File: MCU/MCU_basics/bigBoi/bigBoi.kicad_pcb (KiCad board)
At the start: 2 copper layers, 70 x 70 mm, 90 parts, among them IC1 BMP390, J1 Conn_Coaxial, J2 Conn_Coaxial, J3 DM3AT-SF-PEJM5_40_, J4 Conn_01x05, J5 Conn_01x04, J6 Conn_01x06, J7 USB_B_Micro, SW1 Boot Switch, U1 STM32F469NIHx, U2 LT1963AxST-3.3, U3 SX1276, U5 MIA-M10Q, U6 BNO086, Y1 8MHz, Y3 32kHz

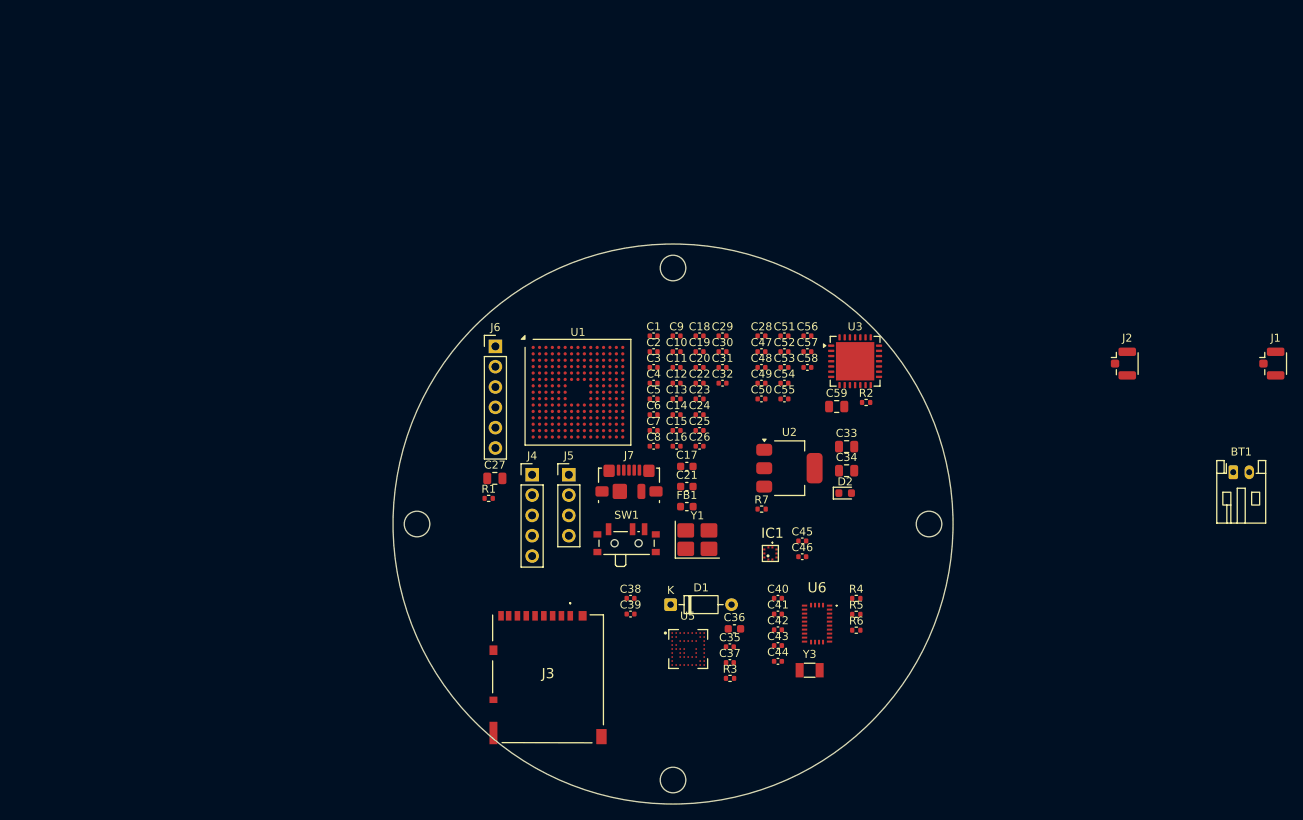
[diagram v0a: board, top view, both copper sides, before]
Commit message: Via escape routing
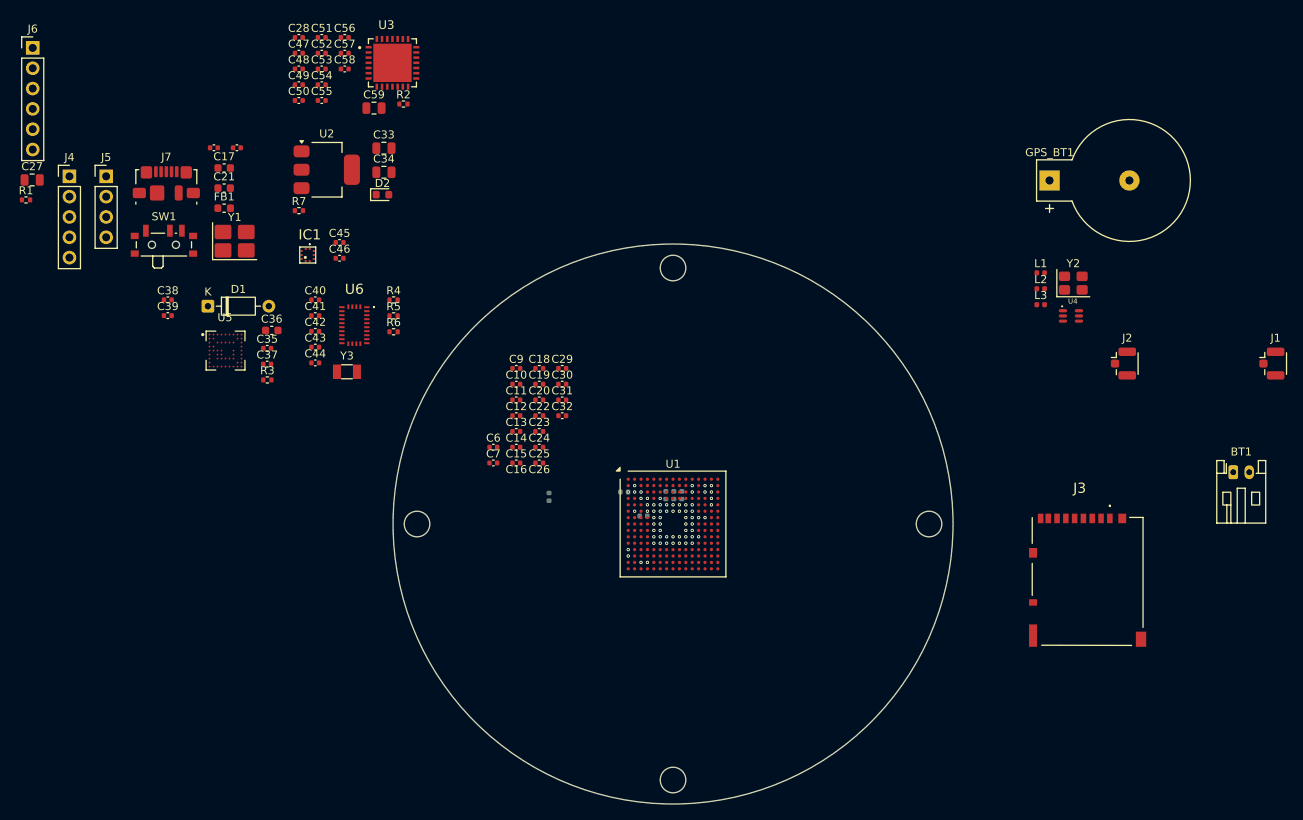
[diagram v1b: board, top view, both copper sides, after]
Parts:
- added GPS_BT1: CR1220, Battery:BatteryHolder_Keystone_500, F.Cu at (155.1, 57.1)
- added L1: 10nH, Inductor_SMD:L_0402_1005Metric, F.Cu at (154.0, 68.6)
- added L2: 10nH, Inductor_SMD:L_0402_1005Metric, F.Cu at (154.0, 70.6)
- added L3: 6.2nH, Inductor_SMD:L_0402_1005Metric, F.Cu at (154.0, 72.6)
- added U4: PE4259, Nebula-footprints:SOT65P215X110-6N, F.Cu at (157.7, 74.0)
- added Y2: 32MHz, Crystal:Crystal_SMD_3225-4Pin_3.2x2.5mm, F.Cu at (158.0, 69.9)
- C1, C2, C3, C4, C5, C8: moved to B.Cu
- C14, C18: value 0402 -> 15pF
- U3: footprint Package_DFN_QFN:QFN-28-1EP_6x6mm_P0.65mm_EP4.8x4.8mm -> Nebula-footprints:QFN65P600X600X100-29N
- moved C28 68.8 mm to (61.2, 39.2)
- moved C47 68.8 mm to (61.2, 41.1)
- moved C48 68.8 mm to (61.2, 43.1)
- moved C56 68.8 mm to (67.0, 39.2)
- moved C57 68.8 mm to (67.0, 41.1)
- moved C58 68.8 mm to (67.0, 43.1)
- moved C59 68.8 mm to (70.6, 48.0)
- moved J4 68.8 mm to (32.5, 56.5)
- moved R4 68.8 mm to (73.1, 72.0)
- moved R6 68.8 mm to (73.1, 76.0)
- moved Y1 68.8 mm to (53.2, 64.6)
- moved Y3 68.8 mm to (67.2, 81.0)
- moved C16 68.8 mm to (50.6, 53.0)
- moved C17 68.8 mm to (51.9, 55.5)
- moved C26 68.8 mm to (53.5, 53.0)
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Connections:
- J3 pad 6: <NO NET> -> GND
- J3 pad MP1: <NO NET> -> GND
- J3 pad MP2: <NO NET> -> GND
- J3 pad MP3: <NO NET> -> GND
- J3 pad MP4: <NO NET> -> GND
- J3 pad MP5: <NO NET> -> GND
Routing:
- net +3.3V: track 0.00 -> 0.24 mm, vias 0 -> 20
- net BNO086_WAKE/PS0_N: track 0.00 -> 0.10 mm, vias 0 -> 1
- net BMP390_CS_N: track 0.00 -> 0.10 mm, vias 0 -> 1
- net GND: track 0.00 -> 0.10 mm, vias 0 -> 22
- net SX1276_SCK_N: vias 0 -> 1
- net SX1276_MISO_N: vias 0 -> 1
- net Net-(U1-VCAP2): vias 0 -> 1
- net Net-(U1-VCAP1): vias 0 -> 1
- net Net-(U1-PDR_ON): vias 0 -> 1
- net Net-(U1-BOOT0): vias 0 -> 1
- net GPS_TX_N: vias 0 -> 1
- net GPS_RX_N: vias 0 -> 1
- net DM3AT_MOSI_0: vias 0 -> 1
- net BNO086_NRST_N: vias 0 -> 1
- net BNO086_INTN_N: vias 0 -> 1
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- added copper zone on In2.Cu, net +3.3V
- added copper zone on In1.Cu, net GND
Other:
- copper layers 2 -> 4
